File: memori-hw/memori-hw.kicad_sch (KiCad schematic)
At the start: 2 parts, among them J1 WeAct Studio 2.9{dblquote} E-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, J2 Seeed Studio Xiao ESP32-C3

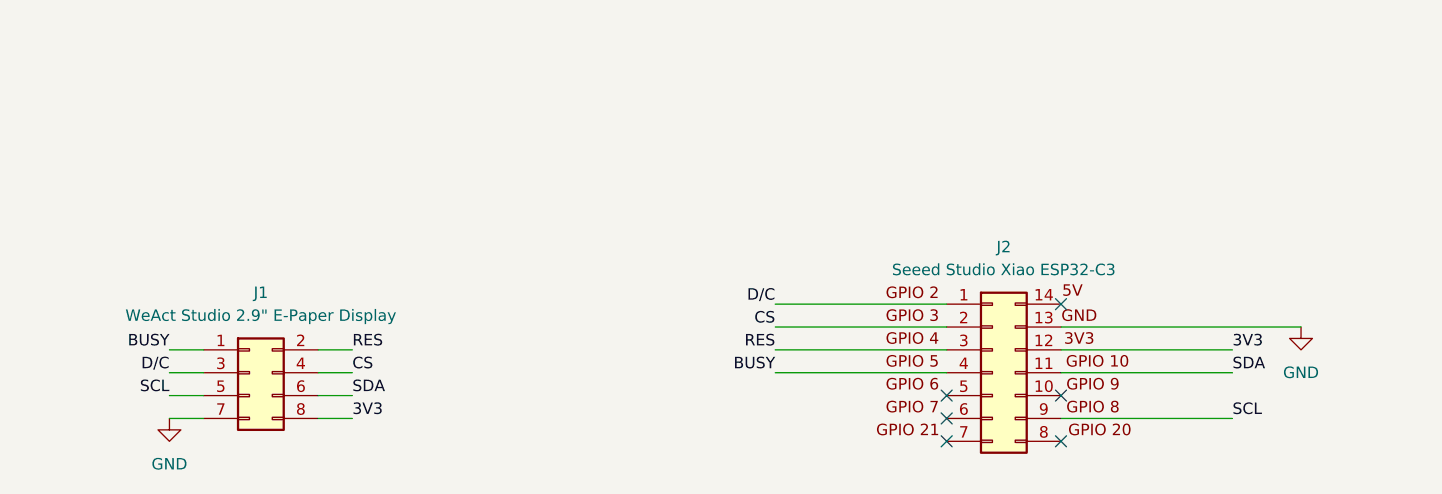
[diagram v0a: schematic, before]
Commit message: feat(hw): Finished battery schematic.
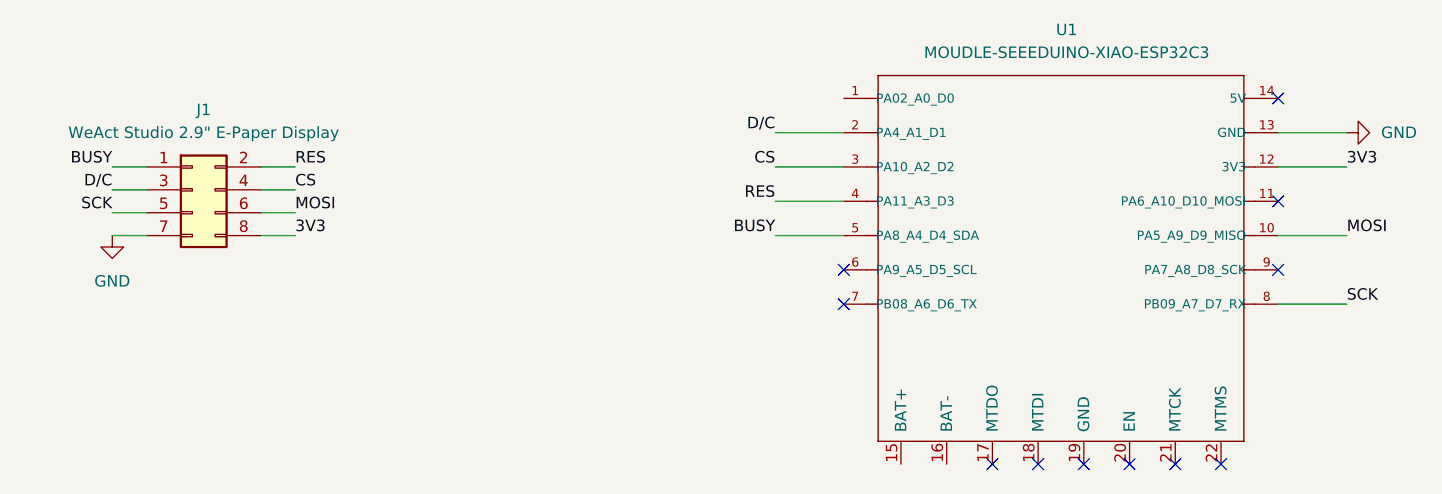
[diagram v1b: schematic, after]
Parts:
- removed J2: Seeed Studio Xiao ESP32-C3, Seeed Studio XIAO Series Library:XIAO-ESP32C3-DIP, symbol Connector_Generic:Conn_02x07_Counter_Clockwise
- added U1: MOUDLE-SEEEDUINO-XIAO-ESP32C3, Seeed Studio XIAO Series Library:XIAO-ESP32C3-SMD, symbol MOUDLE-SEEEDUINO-XIAO-ESP32C3:MOUDLE-SEEEDUINO-XIAO-ESP32C3
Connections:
- net 3V3: now also U1.12 (3V3)
- net BUSY: now also U1.5 (PA8_A4_D4_SDA)
- net CS: now also U1.3 (PA10_A2_D2)
- net D/C: now also U1.2 (PA4_A1_D1)
- net GND: now also U1.13 (GND)
- net RES: now also U1.4 (PA11_A3_D3)
- net SCL renamed SCK
- net SCK: now also U1.8 (PB09_A7_D7_RX)
- net SDA renamed MOSI
- net MOSI: now also U1.10 (PA5_A9_D9_MISO)
- no-connect marks 6 -> 11
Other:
- moved on the sheet: J1
